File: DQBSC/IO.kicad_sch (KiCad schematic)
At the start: 70 parts, among them J1 3-1827253-6, J2 Conn_02x05_Odd_Even, Q1 2SK3018-TP, SW1 SW_DIP_x02, SW2 NANOT160AS, SW3 NANOT160AS, U5 VSC8541XMV-02, Y1 Crystal

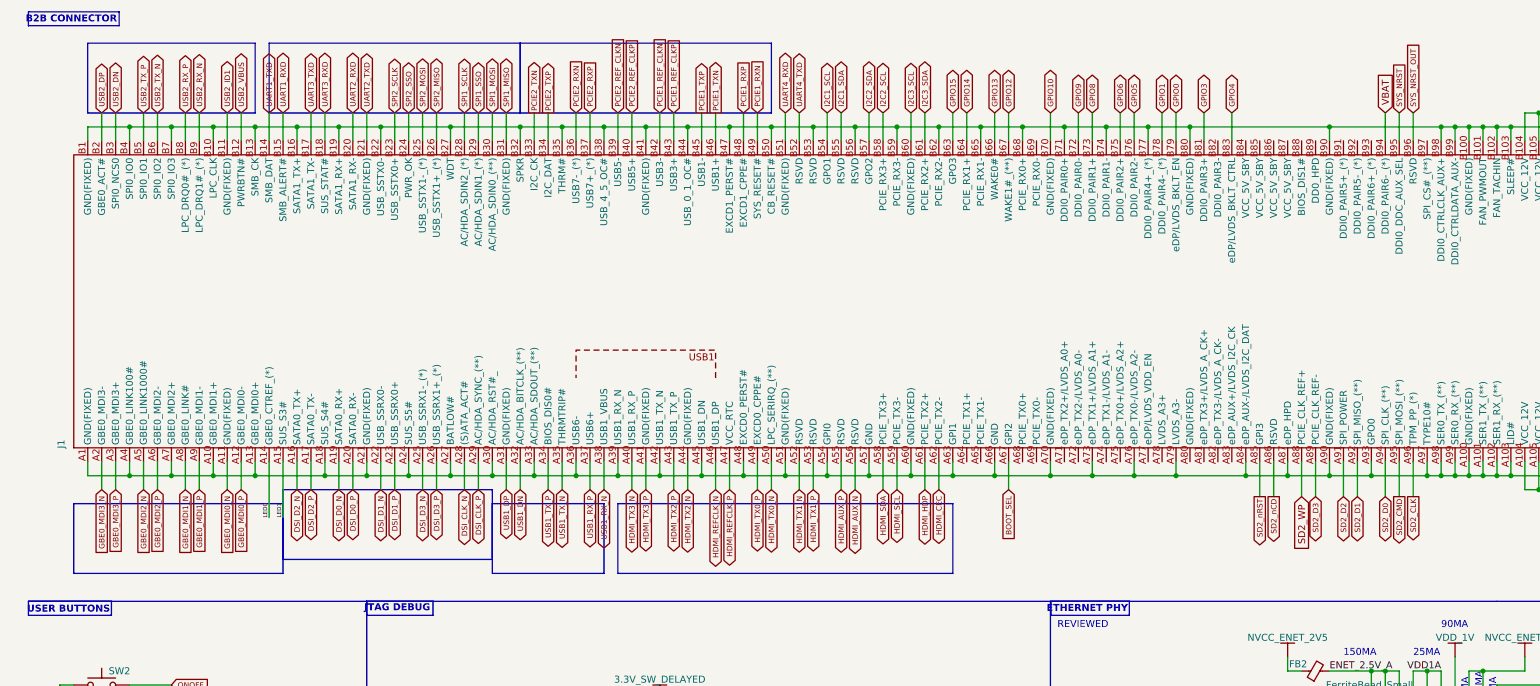
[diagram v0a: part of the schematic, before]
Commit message: Update.
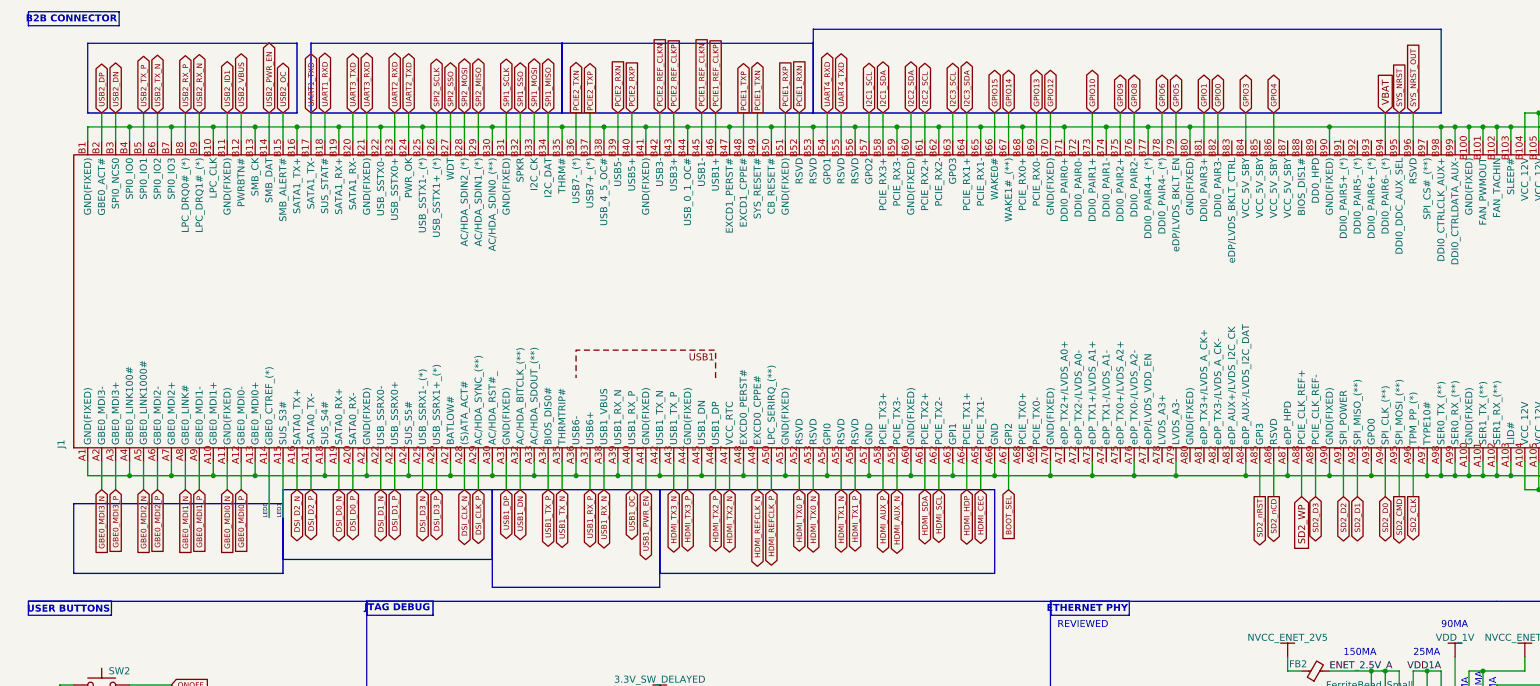
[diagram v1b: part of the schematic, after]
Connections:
- net GND: now also J1.B25 (USB_SSTX1-_(*)), J1.B30 (AC/HDA_SDIN0_(**)); no longer J1.B27 (WDT), J1.B32 (SPKR)
- net GPIO0: now also J1.B82 (DDI0_PAIR3-); no longer J1.B79 (eDP/LVDS_BKLT_EN)
- net GPIO1: now also J1.B81 (DDI0_PAIR3+); no longer J1.B78 (DDI0_PAIR4-_(*))
- net GPIO10: now also J1.B73 (DDI0_PAIR1+); no longer J1.B70 (GND(FIXED))
- net GPIO12: now also J1.B70 (GND(FIXED)); no longer J1.B67 (WAKE1#_(**))
- net GPIO13: now also J1.B69 (PCIE_RX0-); no longer J1.B66 (WAKE0#)
- net GPIO14: now also J1.B67 (WAKE1#_(**)); no longer J1.B64 (PCIE_RX1+)
- net GPIO15: now also J1.B66 (WAKE0#); no longer J1.B63 (GPO3)
- net GPIO3: now also J1.B84 (VCC_5V_SBY); no longer J1.B81 (DDI0_PAIR3+)
- net GPIO4: now also J1.B86 (VCC_5V_SBY); no longer J1.B83 (eDP/LVDS_BKLT_CTRL)
- net GPIO5: now also J1.B79 (eDP/LVDS_BKLT_EN); no longer J1.B76 (DDI0_PAIR2-)
- net GPIO6: now also J1.B78 (DDI0_PAIR4-_(*)); no longer J1.B75 (DDI0_PAIR2+)
- net GPIO8: now also J1.B76 (DDI0_PAIR2-); no longer J1.B73 (DDI0_PAIR1+)
- net GPIO9: now also J1.B75 (DDI0_PAIR2+); no longer J1.B72 (DDI0_PAIR0-)
- net HDMI_AUX_N: now also J1.A59 (PCIE_TX3-); no longer J1.A56 (RSVD)
- net HDMI_AUX_P: now also J1.A58 (PCIE_TX3+); no longer J1.A55 (RSVD)
- net HDMI_CEC: now also J1.A65 (PCIE_TX1-); no longer J1.A62 (PCIE_TX2-)
- net HDMI_HDP: now also J1.A64 (PCIE_TX1+); no longer J1.A61 (PCIE_TX2+)
- net HDMI_REFCLK_N: now also J1.A49 (EXCD0_CPPE#); no longer J1.A46 (USB1_DP)
- net HDMI_REFCLK_P: now also J1.A50 (LPC_SERIRQ_(**)); no longer J1.A47 (VCC_RTC)
- net HDMI_SCL: now also J1.A62 (PCIE_TX2-); no longer J1.A59 (PCIE_TX3-)
- net HDMI_SDA: now also J1.A61 (PCIE_TX2+); no longer J1.A58 (PCIE_TX3+)
- net HDMI_TX0_N: now also J1.A53 (RSVD); no longer J1.A50 (LPC_SERIRQ_(**))
- net HDMI_TX0_P: now also J1.A52 (RSVD); no longer J1.A49 (EXCD0_CPPE#)
- net HDMI_TX1_N: now also J1.A55 (RSVD); no longer J1.A52 (RSVD)
- net HDMI_TX1_P: now also J1.A56 (RSVD); no longer J1.A53 (RSVD)
- net HDMI_TX2_N: now also J1.A47 (VCC_RTC); no longer J1.A44 (GND(FIXED))
- net HDMI_TX2_P: now also J1.A46 (USB1_DP); no longer J1.A43 (USB1_TX_P)
- net HDMI_TX3_N: now also J1.A43 (USB1_TX_P); no longer J1.A40 (USB1_RX_P)
- net HDMI_TX3_P: now also J1.A44 (GND(FIXED)); no longer J1.A41 (GND(FIXED))
- net I2C1_SCL: now also J1.B57 (GPO2); no longer J1.B54 (GPO1)
- net I2C1_SDA: now also J1.B58 (PCIE_RX3+); no longer J1.B55 (RSVD)
- net I2C2_SCL: now also J1.B61 (PCIE_RX2+); no longer J1.B58 (PCIE_RX3+)
- net I2C2_SDA: now also J1.B60 (GND(FIXED)); no longer J1.B57 (GPO2)
- net I2C3_SCL: now also J1.B63 (GPO3); no longer J1.B60 (GND(FIXED))
- net I2C3_SDA: now also J1.B64 (PCIE_RX1+); no longer J1.B61 (PCIE_RX2+)
- net PCIE1_REF_CLKN: now also J1.B45 (USB1-); no longer J1.B42 (USB3-)
- net PCIE1_REF_CLKP: now also J1.B46 (USB1+); no longer J1.B43 (USB3+)
- net PCIE1_RXN: now also J1.B52 (RSVD); no longer J1.B49 (SYS_RESET#)
- net PCIE1_RXP: now also J1.B51 (GND(FIXED)); no longer J1.B48 (EXCD1_CPPE#)
- net PCIE1_TXN: now also J1.B49 (SYS_RESET#); no longer J1.B46 (USB1+)
- net PCIE1_TXP: now also J1.B48 (EXCD1_CPPE#); no longer J1.B45 (USB1-)
- net PCIE2_REF_CLKN: now also J1.B42 (USB3-); no longer J1.B39 (USB5-)
- net PCIE2_REF_CLKP: now also J1.B43 (USB3+); no longer J1.B40 (USB5+)
- net PCIE2_RXN: now also J1.B39 (USB5-); no longer J1.B36 (USB7-_(*))
- net PCIE2_RXP: now also J1.B40 (USB5+); no longer J1.B37 (USB7+_(*))
- net PCIE2_TXN: now also J1.B36 (USB7-_(*)); no longer J1.B33 (I2C_CK)
- net PCIE2_TXP: now also J1.B37 (USB7+_(*)); no longer J1.B34 (I2C_DAT)
- net SPI1_MISO: now also J1.B34 (I2C_DAT); no longer J1.B31 (GND(FIXED))
- net SPI1_MOSI: now also J1.B33 (I2C_CK); no longer J1.B30 (AC/HDA_SDIN0_(**))
- net SPI1_SCLK: now also J1.B31 (GND(FIXED)); no longer J1.B28 (AC/HDA_SDIN2_(*))
- net SPI1_SSO: now also J1.B32 (SPKR); no longer J1.B29 (AC/HDA_SDIN1_(*))
- net SPI2_MISO: now also J1.B29 (AC/HDA_SDIN1_(*)); no longer J1.B26 (USB_SSTX1+_(*))
- net SPI2_MOSI: now also J1.B28 (AC/HDA_SDIN2_(*)); no longer J1.B25 (USB_SSTX1-_(*))
- net SPI2_SCLK: now also J1.B26 (USB_SSTX1+_(*)); no longer J1.B23 (USB_SSTX0+)
- net SPI2_SSO: now also J1.B27 (WDT); no longer J1.B24 (PWR_OK)
- net UART1_RXD: now also J1.B18 (SUS_STAT#); no longer J1.B15 (SMB_ALERT#)
- net UART1_TXD: now also J1.B17 (SATA1_TX-); no longer J1.B14 (SMB_DAT)
- net UART2_RXD: now also J1.B23 (USB_SSTX0+); no longer J1.B20 (SATA1_RX-)
- net UART2_TXD: now also J1.B24 (PWR_OK); no longer J1.B21 (GND(FIXED))
- net UART3_RXD: now also J1.B21 (GND(FIXED)); no longer J1.B18 (SUS_STAT#)
- net UART3_TXD: now also J1.B20 (SATA1_RX-); no longer J1.B17 (SATA1_TX-)
- net UART4_RXD: now also J1.B54 (GPO1); no longer J1.B51 (GND(FIXED))
- net UART4_TXD: now also J1.B55 (RSVD); no longer J1.B52 (RSVD)
- new net USB1_OC: J1.A40 (USB1_RX_P)
- new net USB1_PWR_EN: J1.A41 (GND(FIXED))
- new net USB2_OC: J1.B15 (SMB_ALERT#)
- new net USB2_PWR_EN: J1.B14 (SMB_DAT)
